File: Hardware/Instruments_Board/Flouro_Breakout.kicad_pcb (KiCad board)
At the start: 2 copper layers, 97.8 x 54.9 mm, 52 parts, among them J1 RJ45_LED_Shielded, J2 Conn_01x06_Female, Q1 BSS138, Q10 IRF7606PBF, Q2 BSS138, Q3 IRF7606PBF, Q4 IRF7606PBF, Q5 BSS138, Q6 IRF7606PBF, Q7 BSS138, Q8 IRF7606PBF, Q9 BSS138, U1 Teensy4.1_DEV-16771, U2 3V3 OKI

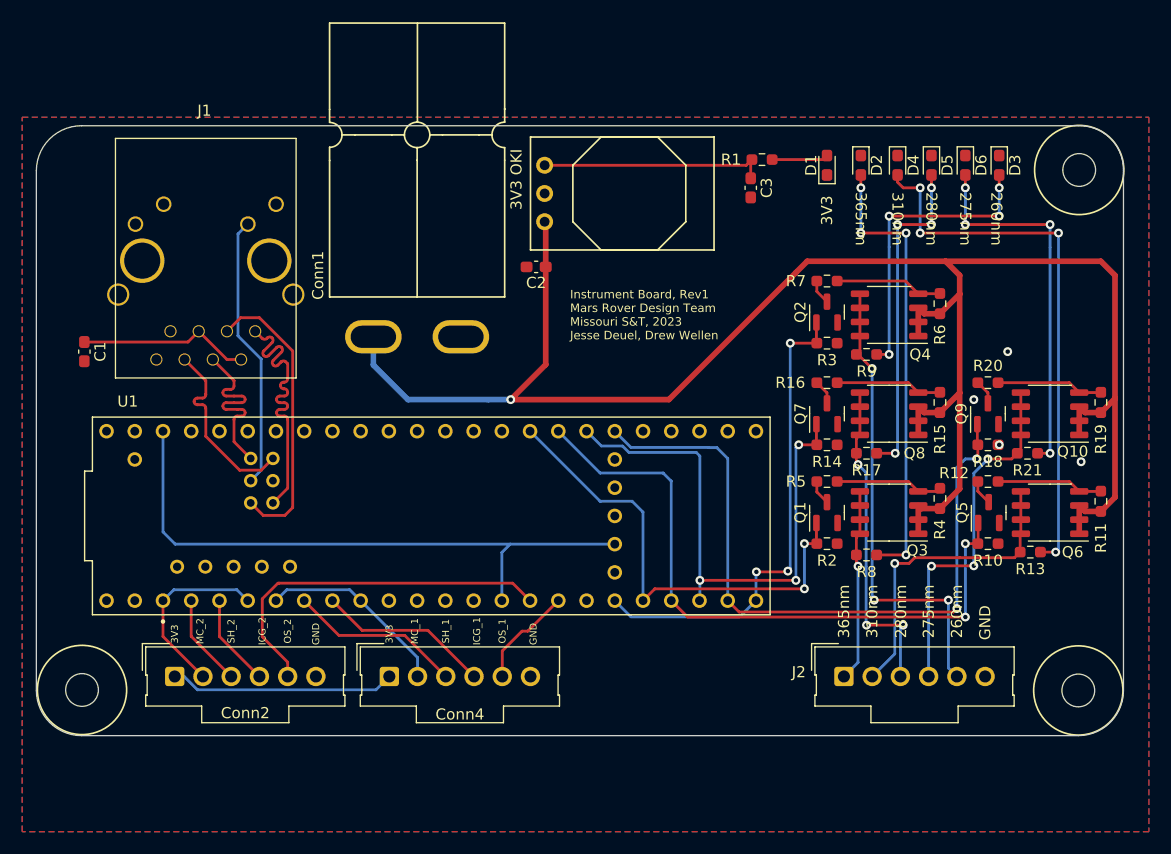
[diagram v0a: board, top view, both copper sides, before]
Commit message: geeeeeerbs
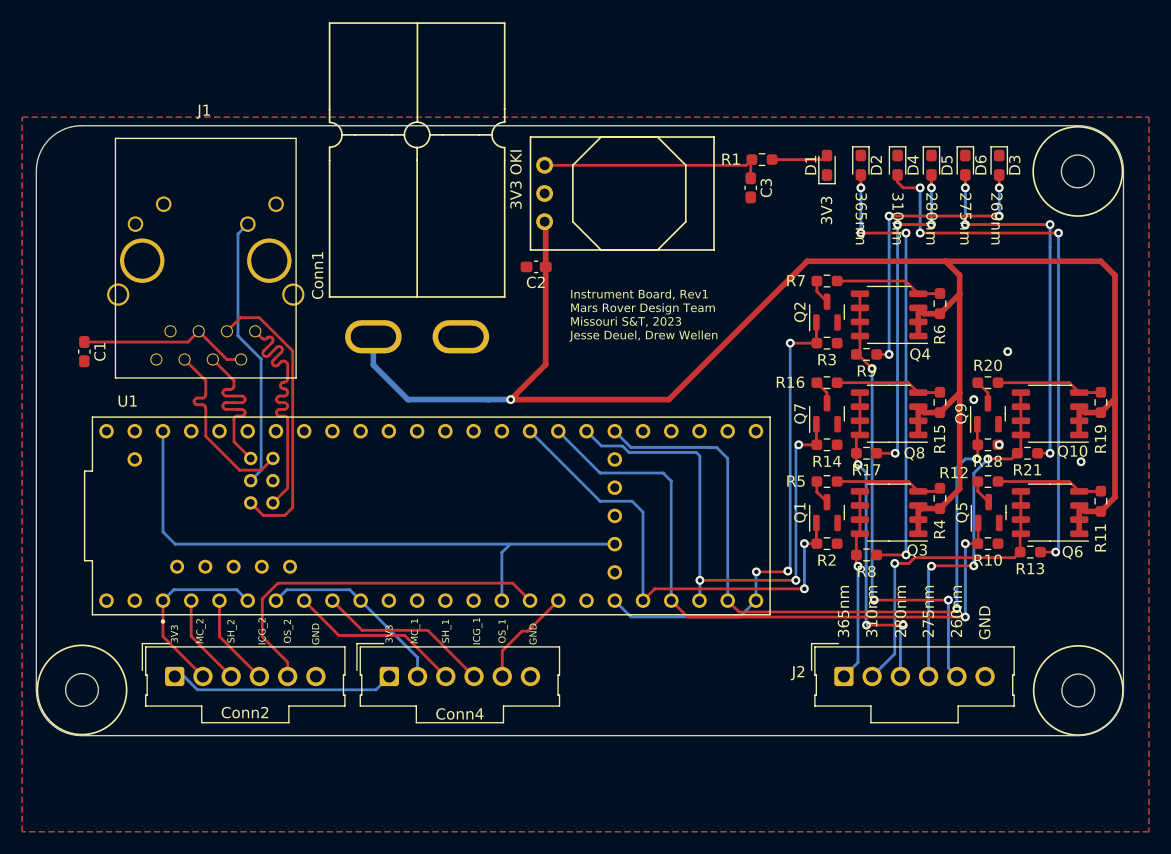
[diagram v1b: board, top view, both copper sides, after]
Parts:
- moved H1 0.18 mm to (197.6, 55.9)
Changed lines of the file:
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@@
       (layerselection 0x00010fc_ffffffff)
       (disableapertmacros false)
-      (usegerberextensions false)
+      (usegerberextensions true)
       (usegerberattributes true)
       (usegerberadvancedattributes true)
@@
       (plotinvisibletext false)
       (sketchpadsonfab false)
-      (subtractmaskfromsilk false)
+      (subtractmaskfromsilk true)
       (outputformat 1)
       (mirror false)
-      (drillshape 1)
+      (drillshape 0)
       (scaleselection 1)
-      (outputdirectory "")
+      (outputdirectory "../../Manufacturing/Gerbs/Sensor_Gerbs/")
     )
   )
@@
   )
   (footprint "MRDT_Drill_Holes:4_40_Hole_Corner" (layer "F.Cu")
-    (at 197.7503 55.7417)
+    (at 197.6233 55.8687)
     (property "Sheetfile" "Flouro_Breakout.kicad_sch")
     (property "Sheetname" "")
@@
     (fp_line (start 15.07 1.79) (end 15.07 -0.24) (layer "F.Fab") (width 0.1))
     (fp_line (start 15.2 1.79) (end 15.07 1.79) (layer "F.Fab") (width 0.1))
-    (pad "1" thru_hole roundrect (at 0 0) (size 1.74 1.74) (drill 1.09) (layers *.Cu *.Mask) (roundrect_rratio 0.143678)
+    (pad "1" thru_hole roundrect (at 0 0) (size 1.74 1.74) (drill 1.09) (layers *.Cu *.Mask) (roundrect_rratio 0.1436781609)
       (net 5 "+3V3") (pintype "input"))
     (pad "2" thru_hole circle (at 2.54 0) (size 1.74 1.74) (drill 1.09) (layers *.Cu *.Mask)
@@
     (fp_line (start 10.16 4.05) (end 10.16 2.55) (layer "F.Fab") (width 0.1))
     (fp_line (start 2.54 2.55) (end 2.54 4.05) (layer "F.Fab") (width 0.1))
-    (pad "1" thru_hole roundrect (at 0 0) (size 1.74 1.74) (drill 1.09) (layers *.Cu *.Mask) (roundrect_rratio 0.143678)
+    (pad "1" thru_hole roundrect (at 0 0) (size 1.74 1.74) (drill 1.09) (layers *.Cu *.Mask) (roundrect_rratio 0.1436781609)
       (net 63 "365nm") (pinfunction "Pin_1") (pintype "passive"))
     (pad "2" thru_hole circle (at 2.54 0) (size 1.74 1.74) (drill 1.09) (layers *.Cu *.Mask)
@@
     (fp_line (start 0.5 -2.55) (end 0 -1.842893) (layer "F.Fab") (width 0.1))
     (fp_line (start 15.2 -0.24) (end 15.2 -2.55) (layer "F.Fab") (width 0.1))
-    (pad "1" thru_hole roundrect (at 0 0) (size 1.74 1.74) (drill 1.09) (layers *.Cu *.Mask) (roundrect_rratio 0.143678)
+    (pad "1" thru_hole roundrect (at 0 0) (size 1.74 1.74) (drill 1.09) (layers *.Cu *.Mask) (roundrect_rratio 0.1436781609)
       (net 5 "+3V3") (pintype "input"))
     (pad "2" thru_hole circle (at 2.54 0) (size 1.74 1.74) (drill 1.09) (layers *.Cu *.Mask)
@@
       ) (layer "B.SilkS") (width 0) (fill solid))
   )
+  (gr_arc (start 201.676 47.752) (mid 204.549682 48.942318) (end 205.74 51.816) (layer "Edge.Cuts") (width 0.1))
   (gr_line (start 201.676 47.752) (end 112.014 47.752) (layer "Edge.Cuts") (width 0.1))
-  (gr_arc (start 201.676 47.752001) (mid 204.588327 48.903673) (end 205.739999 51.816) (layer "Edge.Cuts") (width 0.1))
   (gr_arc (start 107.95 51.816) (mid 109.140318 48.942318) (end 112.014 47.752) (layer "Edge.Cuts") (width 0.1))
   (gr_arc (start 205.74 98.552) (mid 204.549682 101.425682) (end 201.676 102.616) (layer "Edge.Cuts") (width 0.1))
@@
   (segment (start 196.511 81.915) (end 196.511 80.645) (width 0.254) (layer "F.Cu") (net 64))
   (via (at 185.166 87.122) (size 0.8) (drill 0.4) (layers "F.Cu" "B.Cu") (net 64))
-  (segment (start 185.166 87.122) (end 185.039 87.249) (width 0.254) (layer "B.Cu") (net 64))
   (segment (start 185.166 95.262) (end 183.134 97.294) (width 0.254) (layer "B.Cu") (net 64))
   (segment (start 185.166 87.122) (end 185.166 95.262) (width 0.254) (layer "B.Cu") (net 64))
@@
   (segment (start 181.7135 77.216) (end 181.7135 75.8845) (width 0.25) (layer "F.Cu") (net 65))
   (segment (start 182.033 71.755) (end 182.033 73.025) (width 0.25) (layer "F.Cu") (net 65))
-  (segment (start 182.626 92.6745) (end 182.6615 92.71) (width 0.25) (layer "F.Cu") (net 65))
   (segment (start 182.033 74.295) (end 182.033 75.565) (width 0.25) (layer "F.Cu") (net 65))
   (segment (start 181.7135 78.0815) (end 181.864 78.232) (width 0.25) (layer "F.Cu") (net 65))
